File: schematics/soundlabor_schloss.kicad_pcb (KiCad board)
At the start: 2 copper layers, 76.2 x 31.8 mm, 19 parts, among them P1 CONN_01X03, P2 CONN_01X02, P3 CONN_01X02, Q1 Q_NMOS_GDS

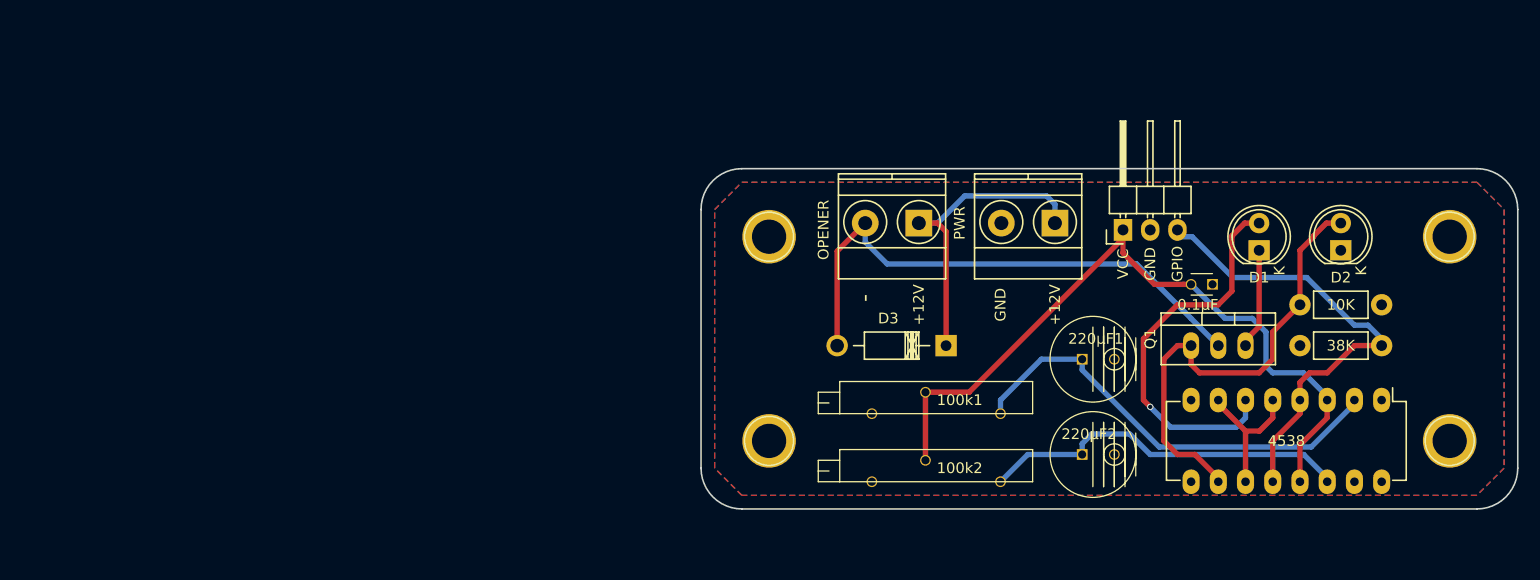
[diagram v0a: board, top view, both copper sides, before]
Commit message: final version
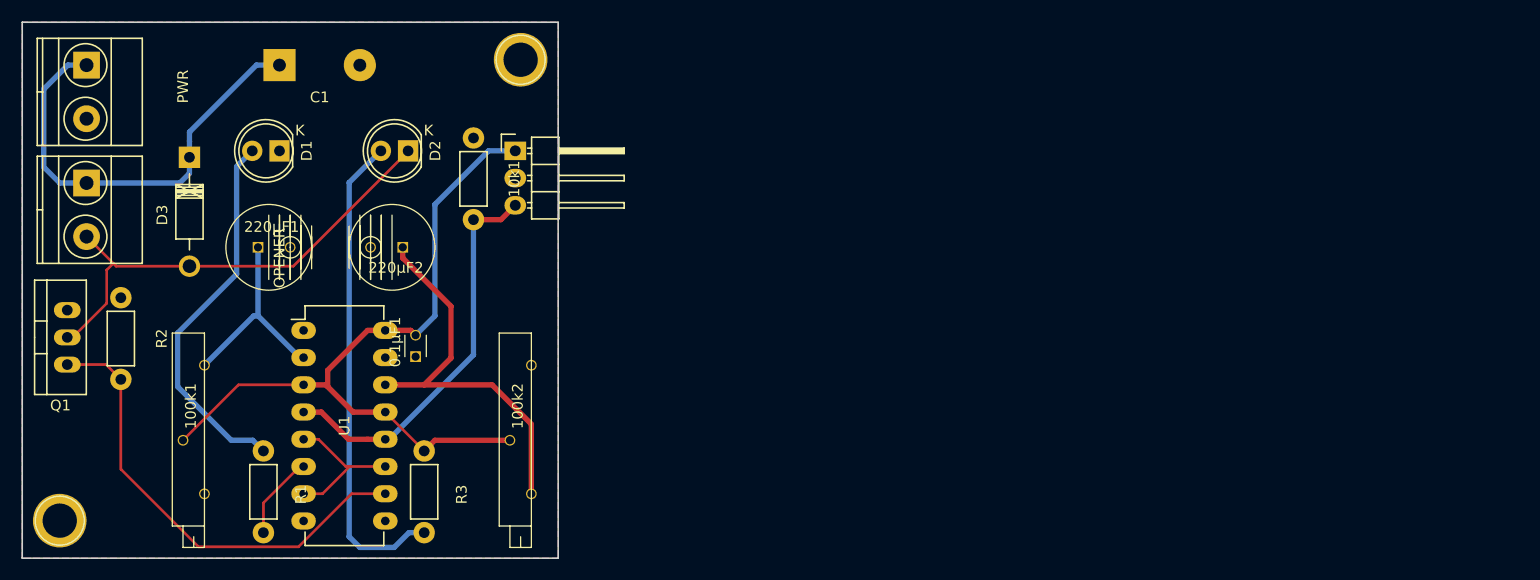
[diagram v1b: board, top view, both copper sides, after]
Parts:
- removed the REF** at (170.2, 80.0)
- removed the REF** at (170.2, 99.1)
- removed the REF** at (106.7, 80.0)
- removed the REF** at (106.7, 99.1)
- added C1: 3300µ, raspberrylock_lib:ECA1EM332, F.Cu at (64.8, 64.0)
- added R1: 120R, Resistors_ThroughHole:Resistor_Horizontal_RM7mm, F.Cu at (59.5, 100.0)
- added R3: 120R, Resistors_ThroughHole:Resistor_Horizontal_RM7mm, F.Cu at (74.5, 100.0)
- added REF**: 1pin, raspberrylock_lib:1pin, F.Cu at (83.5, 63.5)
- added REF**: 1pin, raspberrylock_lib:1pin, F.Cu at (40.5, 106.5)
- R2: renamed from 38K; value 38k -> 100k
- moved R2 117.6 mm to (46.2, 85.7), turned to 270 degrees
- moved Q1 107.4 mm to (41.2, 89.4), turned to 90 degrees
- moved U1 100.8 mm to (63.2, 88.8), turned to 0 degrees
- moved D1 91.9 mm to (61.0, 72.0), turned to 180 degrees
- moved P2 91.5 mm to (43.0, 64.0), turned to 270 degrees
- moved D2 87.5 mm to (73.0, 72.0), turned to 180 degrees
- moved 10k1 79.5 mm to (79.1, 70.8), turned to 270 degrees
- moved P3 77.7 mm to (43.0, 75.0), turned to 270 degrees
- moved 220µF1 77.6 mm to (59.0, 81.0)
- moved 0.1µF1 74.7 mm to (73.7, 91.2), turned to 90 degrees
- moved 100k1 74.4 mm to (54.0, 92.0), turned to 90 degrees
- moved D3 72.7 mm to (52.6, 72.6), turned to 270 degrees
- moved 220µF2 66.3 mm to (72.5, 81.0), turned to 180 degrees
- moved P1 57.2 mm to (83.0, 72.0), turned to 0 degrees
- moved 100k2 45.1 mm to (84.5, 92.0), turned to 90 degrees
- renumbered 0.1µF to 0.1µF1, 10K to 10k1, P3 to P2, P2 to P3, 4538 to U1
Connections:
- net /+12V renamed +12V
- net Net-(10k1-Pad2) renamed PI
- 100k2 pad 1: Net-(100k2-Pad1) -> (no net)
- 100k2 pad 3: (no net) -> Net-(100k2-Pad3)
- 220µF2 pad 1: Net-(100k2-Pad1) -> Net-(100k2-Pad3)
- D2 pad 1: GND -> Net-(D2-Pad1)
- D3 pad 2: Net-(D3-Pad2) -> Net-(D2-Pad1)
- P3 pad 2: Net-(D3-Pad2) -> Net-(D2-Pad1)
- Q1 pad 1: Net-(D2-Pad2) -> Net-(Q1-Pad1)
- Q1 pad 2: Net-(D3-Pad2) -> Net-(D2-Pad1)
- R2 pad 2: Net-(D2-Pad2) -> Net-(Q1-Pad1)
- U1 pad 10: Net-(D2-Pad2) -> Net-(Q1-Pad1)
- U1 pad 14: Net-(100k2-Pad1) -> Net-(100k2-Pad3)
- U1 pad 6: Net-(D1-Pad2) -> Net-(R1-Pad2)
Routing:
- net Net-(D3-Pad2): track 51.7 -> 0.00 mm
- net Net-(D2-Pad1): track 0.00 -> 44.6 mm
- net Net-(Q1-Pad1): track 0.00 -> 43.7 mm
- net Net-(100k2-Pad3): track 0.00 -> 37.4 mm
- net Net-(100k2-Pad1): track 35.0 -> 0.00 mm
- net Net-(100k1-Pad1): track 42.2 -> 19.2 mm
- net +12V: track 29.3 -> 41.5 mm
- net GND: track 9.42 -> 0.00 mm
- net Net-(R1-Pad2): track 0.00 -> 7.93 mm
- net PI: track 43.1 -> 37.2 mm
- net VCC: track 67.9 -> 69.7 mm
- net Net-(D2-Pad2): track 43.9 -> 45.2 mm
- net Net-(D1-Pad2): track 36.6 -> 35.4 mm, vias 1 -> 0
- net Net-(U1-Pad11): track 13.4 -> 14.0 mm
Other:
- board size 76.2 x 31.8 mm -> 50 x 50 mm
- board text added: "c-base door opener anti-schmelz 3000 04/2016"
- board text removed: "+12V"
- board text removed: "-"
- board text removed: "04/2016"
- board text removed: "GND"
- board text removed: "GPIO"
- board text removed: "VCC"
- board text removed: "c-base door opener anti-schmelz 3000"
